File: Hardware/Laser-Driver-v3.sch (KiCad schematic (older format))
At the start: 24 parts, among them J1 Screw_Terminal_01x02, J2 74650074R, J3 74650074R, J4 74650074R, J5 74650074R, Q1 IRFP4568PbF, Q2 PSMN0R7-25YLD, U1 MAX9643, U2 TLV3541

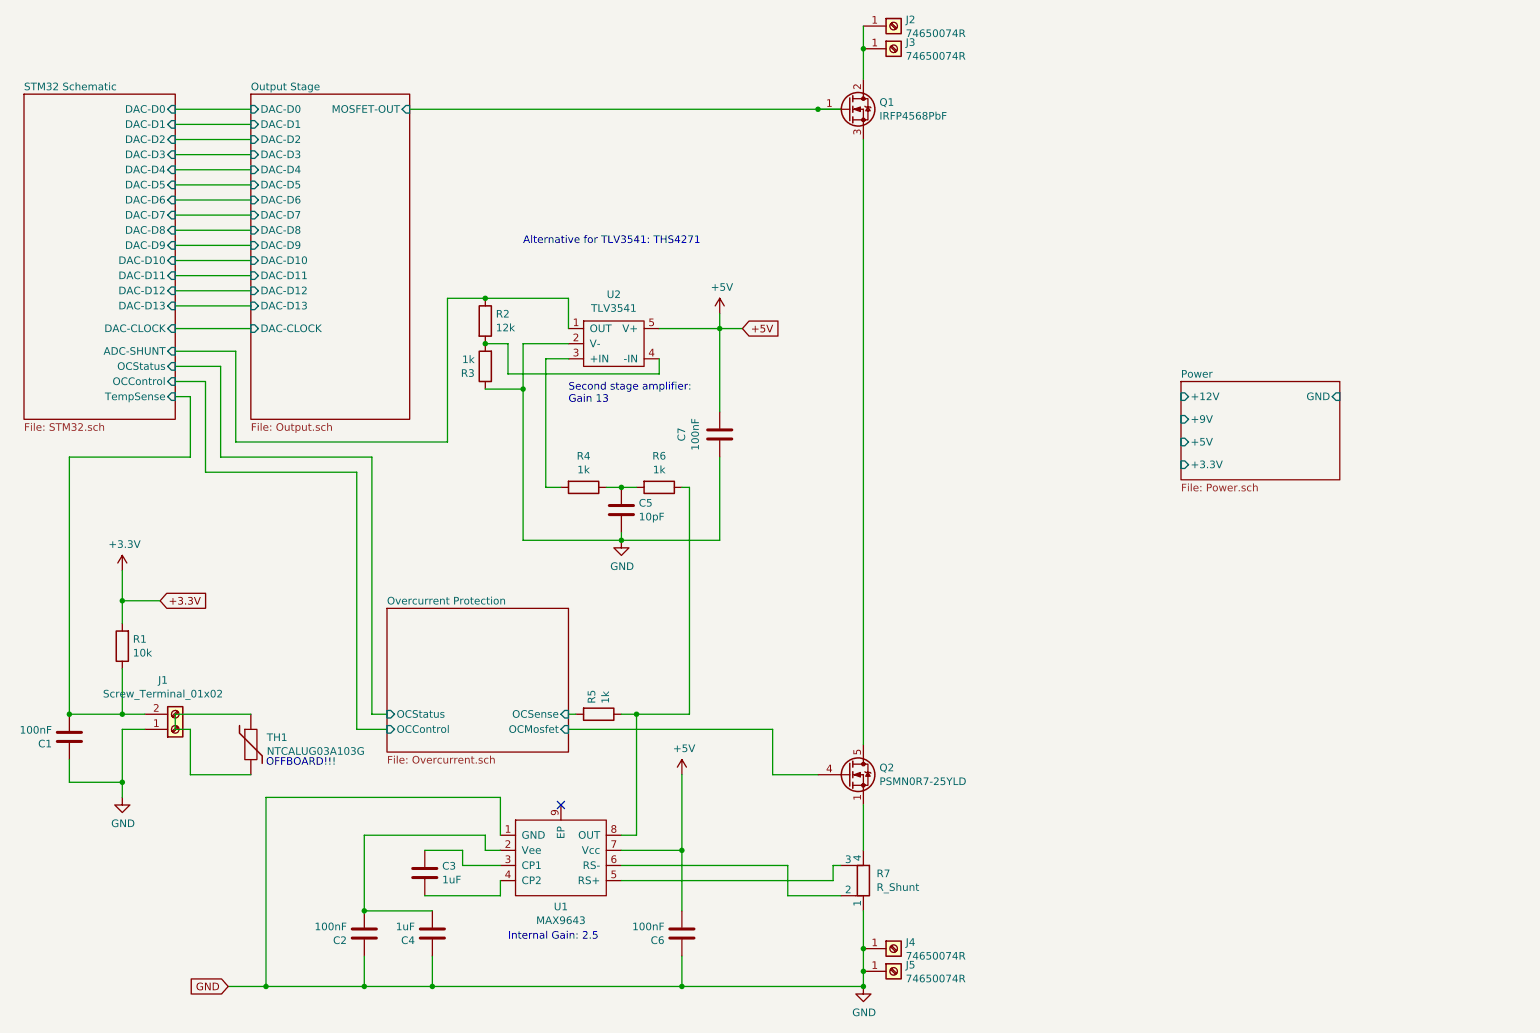
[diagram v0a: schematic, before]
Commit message: STM32 replaced by Teensy
STM32 replaced by Teensy. OPA2354 added as amplifier frontend. Tina-Spice simulation file for amplifier frontend added.
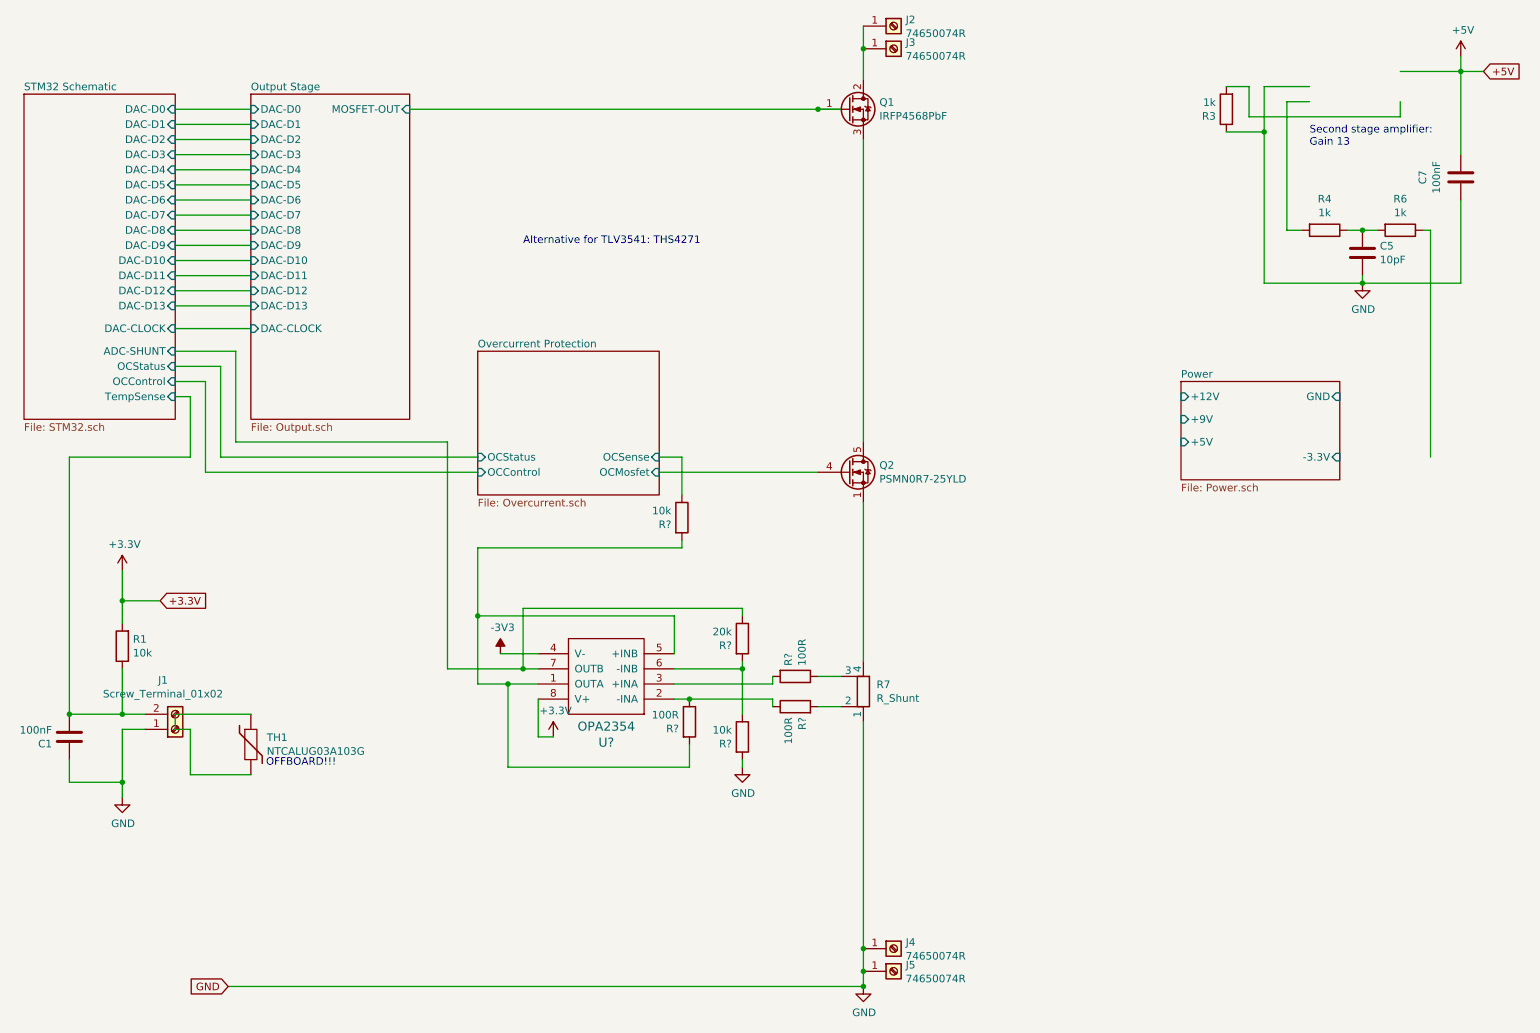
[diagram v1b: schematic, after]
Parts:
- removed C2, C6: 100nF, Capacitor_SMD:C_0603_1608Metric, symbol Device:C
- removed C3, C4: 1uF, Capacitor_SMD:C_0603_1608Metric, symbol Device:C
- removed R2: 12k, Resistor_SMD:R_0603_1608Metric, symbol Device:R
- removed R5: 1k, Resistor_SMD:R_0603_1608Metric, symbol Device:R
- removed U1: MAX9643, symbol OS-LD:MAX9643
- removed U2: TLV3541, Package_TO_SOT_SMD:SOT-23-5, symbol OS-LD:TVL3541
- added R? (x3): 100R, Resistor_SMD:R_0603_1608Metric, symbol Device:R
- added R? (x2): 10k, Resistor_SMD:R_0603_1608Metric, symbol Device:R
- added R?: 20k, Resistor_SMD:R_0603_1608Metric, symbol Device:R
- added U?: OPA2354, symbol OS-LD:OPA2354
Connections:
- net labels added: -3V3
- wire segments 122 -> 111
- no-connect marks 1 -> 0
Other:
- note removed: "Internal Gain: 2.5"
- moved on the sheet: C5, C7, Q2, R3, R4, R6, R7
